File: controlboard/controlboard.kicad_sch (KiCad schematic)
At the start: 25 parts, among them J1 Conn_01x08, J1 Raspberry_Pi_2_3, J2 LimitSwitch, J3 LimitSwitch, J4 LimitSwitch, J5 LimitSwitch, J6 Electromagnet/Servo, J7 Motor, J8 Motor, Q1 TODO, U2 CH224K

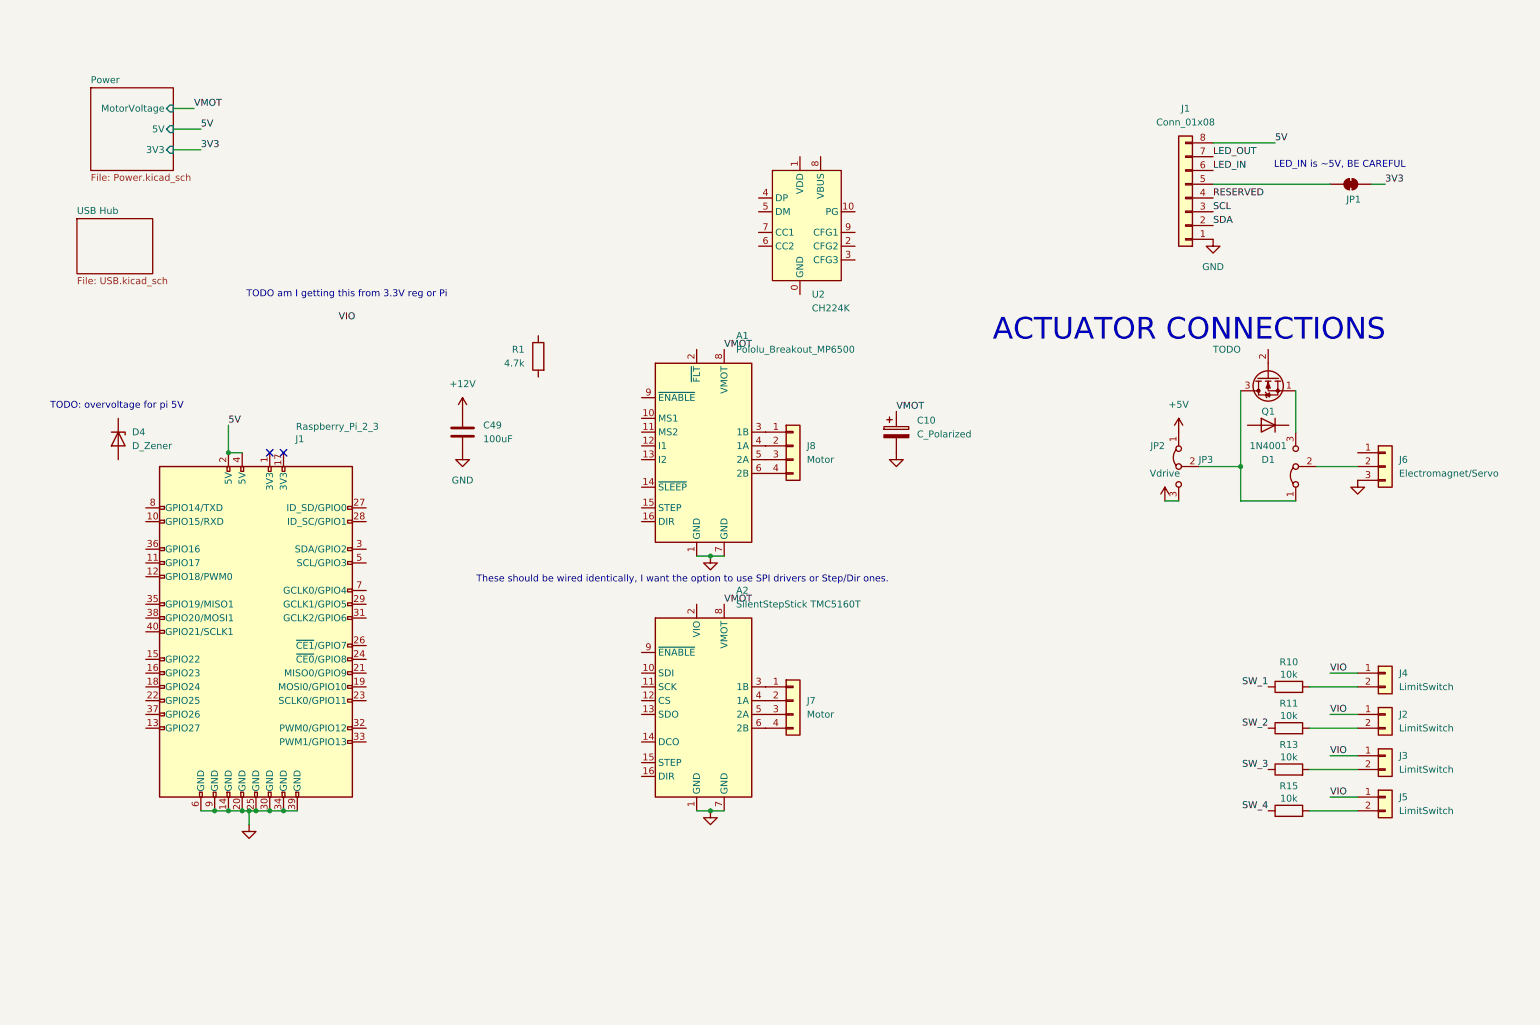
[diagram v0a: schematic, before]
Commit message: Control Board major progress
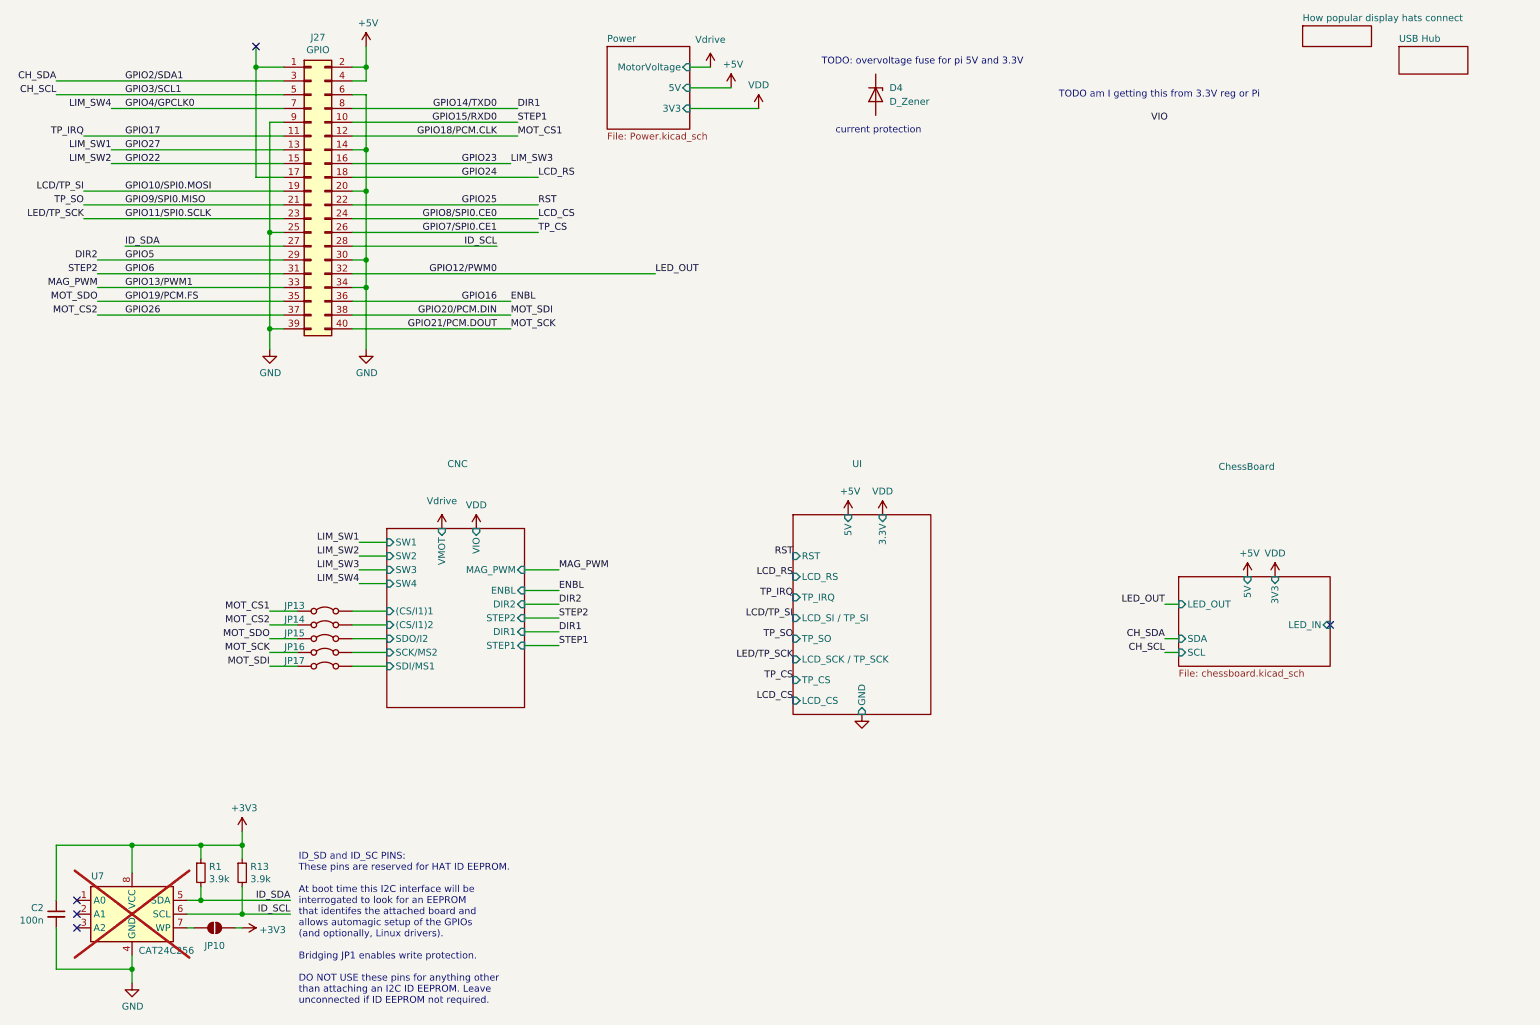
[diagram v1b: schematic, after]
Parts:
- removed A1: Pololu_Breakout_MP6500, Module:Pololu_Breakout-16_15.2x20.3mm, symbol chessbot-parts:Pololu_Breakout_MP6500
- removed A2: SilentStepStick TMC5160T, Module:Pololu_Breakout-16_15.2x20.3mm, symbol chessbot-parts:SilentStepStick
- removed C10: C_Polarized, symbol Device:C_Polarized
- removed C49: 100uF, symbol Device:C
- removed D1: 1N4001, Diode_THT:D_DO-41_SOD81_P10.16mm_Horizontal, symbol Diode:1N4001
- removed J1: Conn_01x08, symbol Connector_Generic:Conn_01x08
- removed J1: Raspberry_Pi_2_3, symbol Connector:Raspberry_Pi_2_3
- removed J2, J3, J4, J5: LimitSwitch, symbol Connector_Generic:Conn_01x02
- removed J6: Electromagnet/Servo, symbol Connector_Generic:Conn_01x03
- removed J7, J8: Motor, symbol Connector_Generic:Conn_01x04
- removed JP1: SolderJumper_2_Bridged, symbol Jumper:SolderJumper_2_Bridged
- removed JP2, JP3: Jumper_3_Bridged12, symbol Jumper:Jumper_3_Bridged12
- removed Q1: TODO, Package_TO_SOT_THT:TO-92_Inline, symbol Transistor_FET:2N7000
- removed R1: 4.7k, symbol Device:R
- removed R10, R11, R13, R15: 10k, symbol Device:R
- removed U2: CH224K, 0my_project:ESSOP-10_CH224K, symbol 0chessbot-parts:CH224K
- added C2: 100n, symbol Device:C_Small
- added J27: GPIO, Connector_PinSocket_2.54mm:PinSocket_2x20_P2.54mm_Vertical, symbol Connector_Generic:Conn_02x20_Odd_Even
- added JP10: ID_WP, symbol Jumper:SolderJumper_2_Open
- added JP13, JP14, JP15, JP16, JP17: Jumper_2_Bridged, symbol Jumper:Jumper_2_Bridged
- added R1, R13: 3.9k, symbol Device:R_Small
- added U7: CAT24C256, symbol Memory_EEPROM:CAT24C256
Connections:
- net +5V: now also J27.2 (Pin_2), J27.4 (Pin_4)
- net GND: now also C2.2, J27.14 (Pin_14), J27.20 (Pin_20), J27.25 (Pin_25), J27.30 (Pin_30), J27.34 (Pin_34), J27.39 (Pin_39), J27.6 (Pin_6), J27.9 (Pin_9), U7.4 (GND)
- new net: JP10.1 (A), U7.7 (WP)
- new net: J27.1 (Pin_1), J27.17 (Pin_17)
- new net +3V3: C2.1, JP10.2 (B), R1.1, R13.1, U7.8 (VCC)
- new net CH_SCL: J27.5 (Pin_5)
- new net CH_SDA: J27.3 (Pin_3)
- new net CNC/(CS/I1)1: JP13.2 (B)
- new net CNC/(CS/I1)2: JP14.2 (B)
- new net CNC/SCK/MS2: JP16.2 (B)
- new net CNC/SDI/MS1: JP17.2 (B)
- new net CNC/SDO/I2: JP15.2 (B)
- new net DIR1: J27.8 (Pin_8)
- new net DIR2: J27.29 (Pin_29)
- new net ENBL: J27.36 (Pin_36)
- new net GPIO10/SPI0.MOSI: J27.19 (Pin_19)
- new net GPIO11/SPI0.SCLK: J27.23 (Pin_23)
- new net GPIO12/PWM0: J27.32 (Pin_32)
- new net GPIO13/PWM1: J27.33 (Pin_33)
- new net GPIO15/RXD0: J27.10 (Pin_10)
- new net GPIO17: J27.11 (Pin_11)
- new net GPIO18/PCM.CLK: J27.12 (Pin_12), JP13.1 (A)
- new net GPIO19/PCM.FS: J27.35 (Pin_35), JP15.1 (A)
- new net GPIO20/PCM.DIN: J27.38 (Pin_38), JP17.1 (A)
- new net GPIO21/PCM.DOUT: J27.40 (Pin_40), JP16.1 (A)
- new net GPIO22: J27.15 (Pin_15)
- new net GPIO23: J27.16 (Pin_16)
- new net GPIO24: J27.18 (Pin_18)
- new net GPIO25: J27.22 (Pin_22)
- new net GPIO26: J27.37 (Pin_37), JP14.1 (A)
- new net GPIO27: J27.13 (Pin_13)
- new net GPIO4/GPCLK0: J27.7 (Pin_7)
- new net GPIO6: J27.31 (Pin_31)
- new net GPIO7/SPI0.CE1: J27.26 (Pin_26)
- new net GPIO8/SPI0.CE0: J27.24 (Pin_24)
- new net GPIO9/SPI0.MISO: J27.21 (Pin_21)
- new net ID_SCL: J27.28 (Pin_28), R13.2, U7.6 (SCL)
- new net ID_SDA: J27.27 (Pin_27), R1.2, U7.5 (SDA)
- no-connect marks 2 -> 5
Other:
- added sheet CNC (cnc.kicad_sch)
- added sheet ChessBoard (chessboard.kicad_sch)
- added sheet How popular display hats connect (display_notes.kicad_sch)
- added sheet UI (ui.kicad_sch)
- note added: "ID_SD and ID_SC PINS: These pins are reserved for HAT ID EEPROM. At boot time this I2C interface will be interrogated to look for an EEPROM that identifes the attached board and allows automagic setup of the GPIOs (and optionally, Linux drivers). Bridging JP1 enables write protection. DO NOT USE these pins for anything other than attaching an I2C ID EEPROM. Leave unconnected if ID EEPROM not requ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"
- note added: "TODO: overvoltage fuse for pi 5V and 3.3V"
- note added: "current protection"
- note removed: "ACTUATOR CONNECTIONS"
- note removed: "LED_IN is ~5V, BE CAREFUL"
- note removed: "TODO: overvoltage for pi 5V"
- note removed: "These should be wired identically, I want the option to use SPI drivers or Step/Dir ones."
- moved on the sheet: D4
